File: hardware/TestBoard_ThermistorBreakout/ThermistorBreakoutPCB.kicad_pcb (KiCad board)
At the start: 2 copper layers, 24.8 x 22.2 mm, 15 parts, among them J1 Conn_01x02, J2 Conn_01x03, J8 Conn_01x06

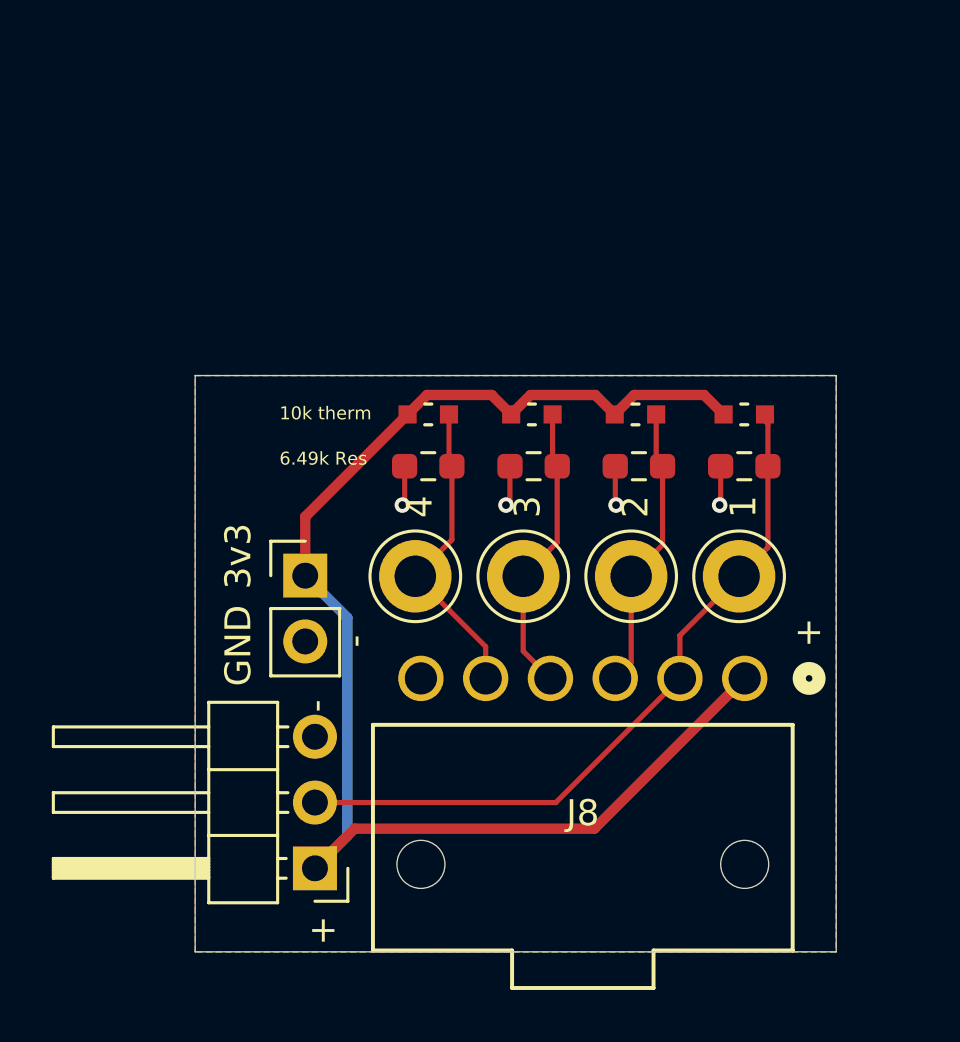
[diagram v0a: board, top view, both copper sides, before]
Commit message: redid thermistor board
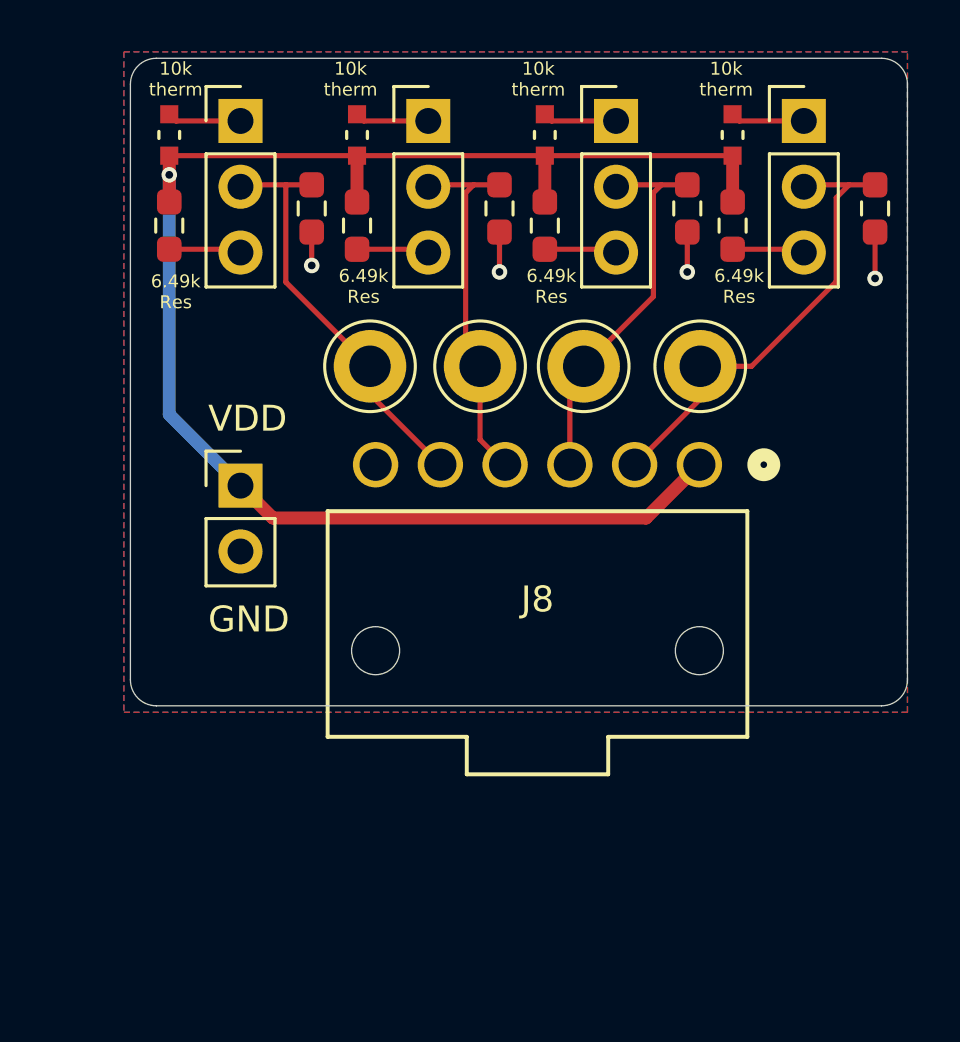
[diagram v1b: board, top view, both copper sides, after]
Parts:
- removed J2: Conn_01x03, Connector_PinHeader_2.54mm:PinHeader_1x03_P2.54mm_Horizontal
- removed R1, R2, R3, R4: 6.49k, Resistor_SMD:R_0603_1608Metric_Pad0.98x0.95mm_HandSolder
- removed TH1, TH2, TH3, TH4: Thermistor_NTC, UTSVT_Special:THERM_ERT-J1VR104FM
- removed TP1, TP2, TP3, TP4: TestPoint, TestPoint:TestPoint_Keystone_5005-5009_Compact
- added J3: Conn_01x03, Connector_PinHeader_2.54mm:PinHeader_1x03_P2.54mm_Vertical, F.Cu at (131.2, 40.2)
- added J4: Conn_01x03, Connector_PinHeader_2.54mm:PinHeader_1x03_P2.54mm_Vertical, F.Cu at (124.0, 40.2)
- added J5: Conn_01x03, Connector_PinHeader_2.54mm:PinHeader_1x03_P2.54mm_Vertical, F.Cu at (116.8, 40.2)
- added J6: Conn_01x03, Connector_PinHeader_2.54mm:PinHeader_1x03_P2.54mm_Vertical, F.Cu at (109.5, 40.2)
- added R10: 6.49k, Resistor_SMD:R_0603_1608Metric_Pad0.98x0.95mm_HandSolder, F.Cu at (112.2, 43.5)
- added R11: 6.49k, Resistor_SMD:R_0603_1608Metric_Pad0.98x0.95mm_HandSolder, F.Cu at (114.0, 44.2)
- added R12: 6.49k, Resistor_SMD:R_0603_1608Metric_Pad0.98x0.95mm_HandSolder, F.Cu at (106.8, 44.2)
- added R5: 6.49k, Resistor_SMD:R_0603_1608Metric_Pad0.98x0.95mm_HandSolder, F.Cu at (128.5, 44.2)
- added R6: 6.49k, Resistor_SMD:R_0603_1608Metric_Pad0.98x0.95mm_HandSolder, F.Cu at (134.0, 43.5)
- added R7: 6.49k, Resistor_SMD:R_0603_1608Metric_Pad0.98x0.95mm_HandSolder, F.Cu at (126.8, 43.5)
- added R8: 6.49k, Resistor_SMD:R_0603_1608Metric_Pad0.98x0.95mm_HandSolder, F.Cu at (121.2, 44.2)
- added R9: 6.49k, Resistor_SMD:R_0603_1608Metric_Pad0.98x0.95mm_HandSolder, F.Cu at (119.5, 43.5)
- added TH5: Thermistor_NTC, UTSVT_Special:THERM_ERT-J1VR104FM, F.Cu at (128.5, 40.7)
- added TH6: Thermistor_NTC, UTSVT_Special:THERM_ERT-J1VR104FM, F.Cu at (121.2, 40.7)
- added TH7: Thermistor_NTC, UTSVT_Special:THERM_ERT-J1VR104FM, F.Cu at (114.0, 40.7)
- added TH8: Thermistor_NTC, UTSVT_Special:THERM_ERT-J1VR104FM, F.Cu at (106.8, 40.7)
- added TP10: TestPoint, TestPoint:TestPoint_Keystone_5005-5009_Compact, F.Cu at (122.8, 49.6)
- added TP11: TestPoint, TestPoint:TestPoint_Keystone_5005-5009_Compact, F.Cu at (127.2, 49.6)
- added TP8: TestPoint, TestPoint:TestPoint_Keystone_5005-5009_Compact, F.Cu at (118.8, 49.6)
- added TP9: TestPoint, TestPoint:TestPoint_Keystone_5005-5009_Compact, F.Cu at (114.5, 49.6)
- moved J8 8.43 mm to (127.2, 53.4)
- moved J1 4.28 mm to (109.5, 54.2)
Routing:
- net /Temperature1: track 27.7 -> 19.3 mm
- net VDDA: track 54.0 -> 61.1 mm, vias 0 -> 1
- net /Temperature2: track 11.1 -> 16.2 mm
- net /Temperature4: track 11.9 -> 16.1 mm
- net /Temperature3: track 11.2 -> 14.3 mm
- net Net-(J3-Pin_1): track 0.00 -> 2.86 mm
- net Net-(J6-Pin_1): track 0.00 -> 2.86 mm
- net Net-(J5-Pin_1): track 0.00 -> 2.86 mm
- net Net-(J4-Pin_1): track 0.00 -> 2.86 mm
- net Net-(J6-Pin_3): track 0.00 -> 2.80 mm
- net Net-(J5-Pin_3): track 0.00 -> 2.80 mm
- net Net-(J4-Pin_3): track 0.00 -> 2.80 mm
- net Net-(J3-Pin_3): track 0.00 -> 2.80 mm
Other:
- board size 24.8 x 22.2 mm -> 30 x 25 mm
- board text added: "VDD"
- board text removed: "+"
- board text removed: "-"
- board text removed: "1"
- board text removed: "2"
- board text removed: "3"
- board text removed: "3v3"
- board text removed: "4"
